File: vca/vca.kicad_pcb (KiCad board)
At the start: 2 copper layers, 68.6 x 101.6 mm, 27 parts, among them J1 Conn_01x02_Socket, J2 Conn_01x02_Socket, J3 Conn_01x02_Socket, J5 Conn_01x03_Socket, Q1 BC548C, Q2 BC548C, U1 TL074

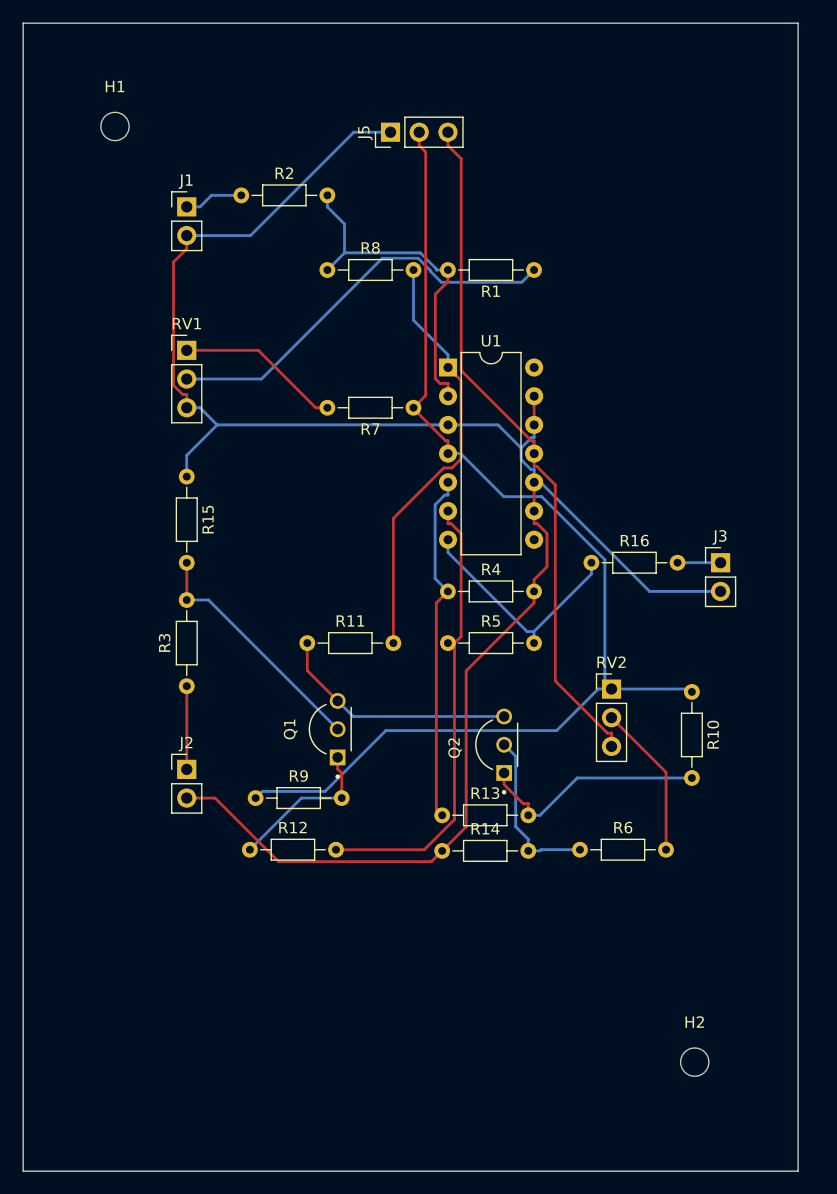
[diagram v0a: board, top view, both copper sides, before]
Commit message: add vco remove zips
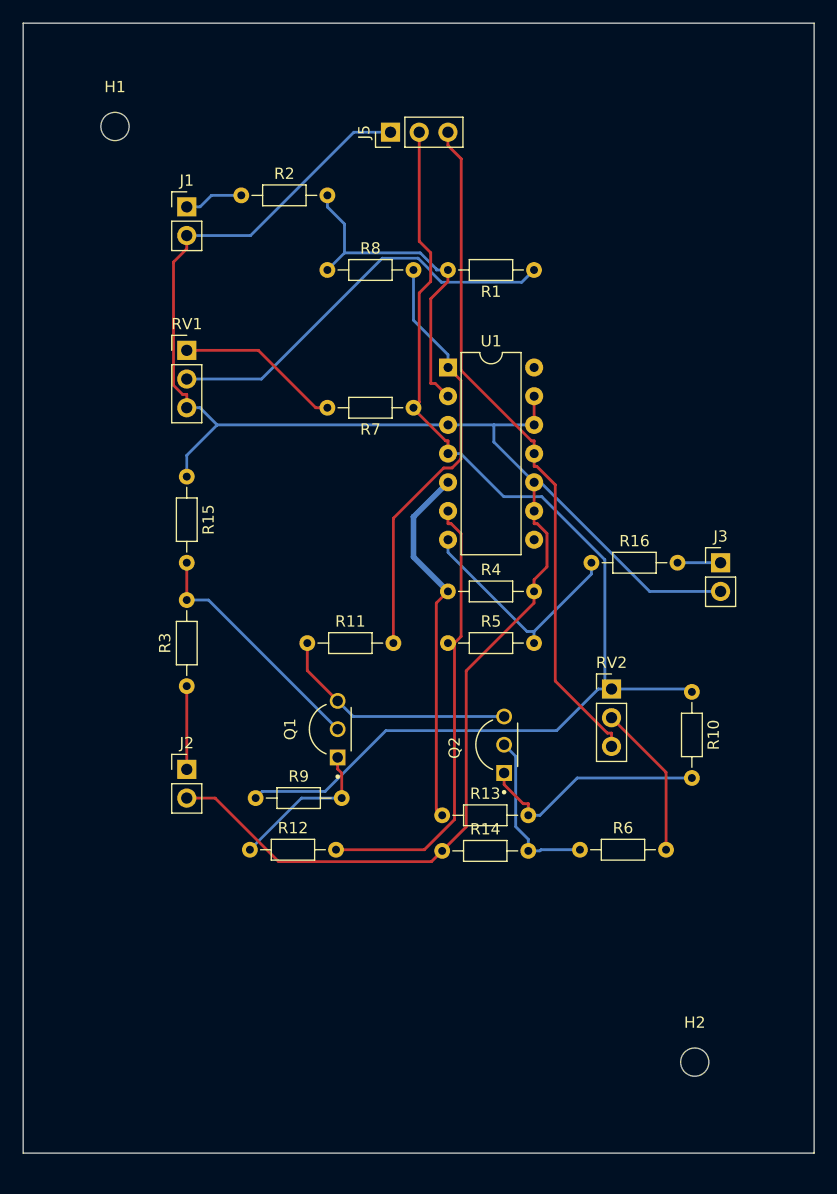
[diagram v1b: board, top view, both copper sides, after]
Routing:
- net Net-(U1B-+): track 31.2 -> 32.6 mm
- net GND: track 167.0 -> 168.1 mm
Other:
- board size 68.6 x 101.6 mm -> 70 x 100 mm
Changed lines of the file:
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@@
     )
   )
-  (gr_rect (start 76.916 22.352) (end 145.496 123.952)
+  (gr_rect (start 76.916 22.352) (end 146.916 122.352)
     (stroke (width 0.1) (type default)) (fill none) (layer "Edge.Cuts"))
   (segment (start 96.22 37.592) (end 93.5869 37.592) (width 0.25) (layer "B.Cu") (net 1))
@@
   (segment (start 92.5709 56.388) (end 94.0899 57.907) (width 0.25) (layer "B.Cu") (net 2))
   (segment (start 91.394 60.6029) (end 91.394 62.484) (width 0.25) (layer "B.Cu") (net 2))
-  (segment (start 121.9045 59.0339) (end 122.138 59.0339) (width 0.25) (layer "B.Cu") (net 2))
-  (segment (start 114.518 57.907) (end 118.9458 57.907) (width 0.25) (layer "B.Cu") (net 2))
   (segment (start 91.394 56.388) (end 92.5709 56.388) (width 0.25) (layer "B.Cu") (net 2))
-  (segment (start 120.9886 60.9924) (end 120.9886 59.9498) (width 0.25) (layer "B.Cu") (net 2))
-  (segment (start 122.138 61.8601) (end 121.8563 61.8601) (width 0.25) (layer "B.Cu") (net 2))
+  (segment (start 118.572 59.421) (end 122.138 62.987) (width 0.25) (layer "B.Cu") (net 2))
+  (segment (start 118.572 57.907) (end 118.572 59.421) (width 0.25) (layer "B.Cu") (net 2))
   (segment (start 106.1828 32.004) (end 97.0388 41.148) (width 0.25) (layer "B.Cu") (net 2))
-  (segment (start 122.138 62.4235) (end 122.138 61.8601) (width 0.25) (layer "B.Cu") (net 2))
   (segment (start 109.428 32.004) (end 106.1828 32.004) (width 0.25) (layer "B.Cu") (net 2))
   (segment (start 138.638 72.644) (end 132.3585 72.644) (width 0.25) (layer "B.Cu") (net 2))
   (segment (start 94.0899 57.907) (end 114.518 57.907) (width 0.25) (layer "B.Cu") (net 2))
-  (segment (start 121.8563 61.8601) (end 120.9886 60.9924) (width 0.25) (layer "B.Cu") (net 2))
-  (segment (start 120.9886 59.9498) (end 121.9045 59.0339) (width 0.25) (layer "B.Cu") (net 2))
+  (segment (start 118.572 57.907) (end 122.138 57.907) (width 0.25) (layer "B.Cu") (net 2))
   (segment (start 122.138 62.987) (end 122.138 62.4235) (width 0.25) (layer "B.Cu") (net 2))
   (segment (start 132.3585 72.644) (end 122.138 62.4235) (width 0.25) (layer "B.Cu") (net 2))
-  (segment (start 122.138 57.907) (end 122.138 59.0339) (width 0.25) (layer "B.Cu") (net 2))
   (segment (start 94.0899 57.907) (end 91.394 60.6029) (width 0.25) (layer "B.Cu") (net 2))
-  (segment (start 118.9458 57.907) (end 120.9886 59.9498) (width 0.25) (layer "B.Cu") (net 2))
+  (segment (start 114.518 57.907) (end 118.572 57.907) (width 0.25) (layer "B.Cu") (net 2))
   (segment (start 104.749 88.3629) (end 105.11 88.7239) (width 0.25) (layer "F.Cu") (net 3))
   (segment (start 105.11 88.7239) (end 105.11 90.932) (width 0.25) (layer "F.Cu") (net 3))
@@
   (segment (start 111.8687 43.1525) (end 112.984 44.2678) (width 0.25) (layer "B.Cu") (net 8))
   (segment (start 112.984 44.34) (end 113.9246 45.2806) (width 0.25) (layer "B.Cu") (net 8))
-  (segment (start 113.3911 46.3398) (end 114.508 45.2229) (width 0.25) (layer "F.Cu") (net 9))
-  (segment (start 113.8136 54.2401) (end 113.3911 53.8176) (width 0.25) (layer "F.Cu") (net 9))
-  (segment (start 114.518 55.367) (end 114.518 54.2401) (width 0.25) (layer "F.Cu") (net 9))
-  (segment (start 114.508 44.196) (end 114.508 45.2229) (width 0.25) (layer "F.Cu") (net 9))
-  (segment (start 114.518 54.2401) (end 113.8136 54.2401) (width 0.25) (layer "F.Cu") (net 9))
-  (segment (start 113.3911 53.8176) (end 113.3911 46.3398) (width 0.25) (layer "F.Cu") (net 9))
+  (segment (start 114.508 45.2229) (end 114.508 44.196) (width 0.25) (layer "F.Cu") (net 9))
+  (segment (start 112.9895 46.7414) (end 114.508 45.2229) (width 0.25) (layer "F.Cu") (net 9))
+  (segment (start 112.9895 54.2401) (end 112.9895 46.7414) (width 0.25) (layer "F.Cu") (net 9))
+  (segment (start 112.9895 54.2401) (end 113.3911 54.2401) (width 0.25) (layer "F.Cu") (net 9))
+  (segment (start 113.3911 54.2401) (end 114.518 55.367) (width 0.25) (layer "F.Cu") (net 9))
   (segment (start 112.0566 42.6825) (end 105.3535 42.6825) (width 0.25) (layer "B.Cu") (net 9))
   (segment (start 113.4811 44.107) (end 112.0566 42.6825) (width 0.25) (layer "B.Cu") (net 9))
@@
   (segment (start 114.508 72.644) (end 113.4804 73.6716) (width 0.25) (layer "F.Cu") (net 11))
   (segment (start 113.4804 91.9364) (end 114 92.456) (width 0.25) (layer "F.Cu") (net 11))
-  (segment (start 113.3754 71.5114) (end 114.508 72.644) (width 0.25) (layer "B.Cu") (net 11))
-  (segment (start 113.3754 64.9748) (end 113.3754 71.5114) (width 0.25) (layer "B.Cu") (net 11))
-  (segment (start 114.518 62.987) (end 114.518 64.1139) (width 0.25) (layer "B.Cu") (net 11))
-  (segment (start 114.2363 64.1139) (end 113.3754 64.9748) (width 0.25) (layer "B.Cu") (net 11))
-  (segment (start 114.518 64.1139) (end 114.2363 64.1139) (width 0.25) (layer "B.Cu") (net 11))
+  (segment (start 111.46 69.596) (end 114.508 72.644) (width 0.5) (layer "B.Cu") (net 11))
+  (segment (start 114.518 62.987) (end 111.465 66.04) (width 0.5) (layer "B.Cu") (net 11))
+  (segment (start 111.465 66.04) (end 111.46 66.04) (width 0.5) (layer "B.Cu") (net 11))
+  (segment (start 111.46 66.04) (end 111.46 69.596) (width 0.5) (layer "B.Cu") (net 11))
   (segment (start 114.518 66.6539) (end 114.7997 66.6539) (width 0.25) (layer "F.Cu") (net 12))
   (segment (start 115.6726 76.6337) (end 115.0903 77.216) (width 0.25) (layer "F.Cu") (net 12))
@@
   (segment (start 133.812 88.646) (end 133.812 95.504) (width 0.25) (layer "F.Cu") (net 14))
   (segment (start 114.518 59.3201) (end 114.3141 59.3201) (width 0.25) (layer "F.Cu") (net 15))
-  (segment (start 111.968 32.004) (end 111.968 33.1809) (width 0.25) (layer "F.Cu") (net 15))
-  (segment (start 112.5395 55.3085) (end 111.46 56.388) (width 0.25) (layer "F.Cu") (net 15))
-  (segment (start 112.5395 33.7524) (end 112.5395 55.3085) (width 0.25) (layer "F.Cu") (net 15))
+  (segment (start 111.968 46.228) (end 111.968 55.88) (width 0.25) (layer "F.Cu") (net 15))
+  (segment (start 111.968 46.228) (end 112.984 45.212) (width 0.25) (layer "F.Cu") (net 15))
+  (segment (start 112.984 42.672) (end 111.968 41.656) (width 0.25) (layer "F.Cu") (net 15))
+  (segment (start 111.968 55.88) (end 111.46 56.388) (width 0.25) (layer "F.Cu") (net 15))
+  (segment (start 112.984 45.212) (end 112.984 42.672) (width 0.25) (layer "F.Cu") (net 15))
   (segment (start 114.3141 59.3201) (end 111.46 56.466) (width 0.25) (layer "F.Cu") (net 15))
-  (segment (start 111.968 33.1809) (end 112.5395 33.7524) (width 0.25) (layer "F.Cu") (net 15))
+  (segment (start 111.968 32.004) (end 111.968 41.656) (width 0.25) (layer "F.Cu") (net 15))
   (segment (start 111.46 56.466) (end 111.46 56.388) (width 0.25) (layer "F.Cu") (net 15))
   (segment (start 114.518 60.447) (end 114.518 59.3201) (width 0.25) (layer "F.Cu") (net 15))
